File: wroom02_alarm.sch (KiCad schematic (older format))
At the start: 29 parts, among them J1 Serial, J10 pin, J11 pin, J2 BARREL_JACK, J3 microUSB, J4 pin, J5 pin, J6 pin, J7 pin, J8 pin, J9 pin, Q1 Q_NMOS_GDS, SW1 Write, SW2 RESET, U1 wroom02, U3 7803

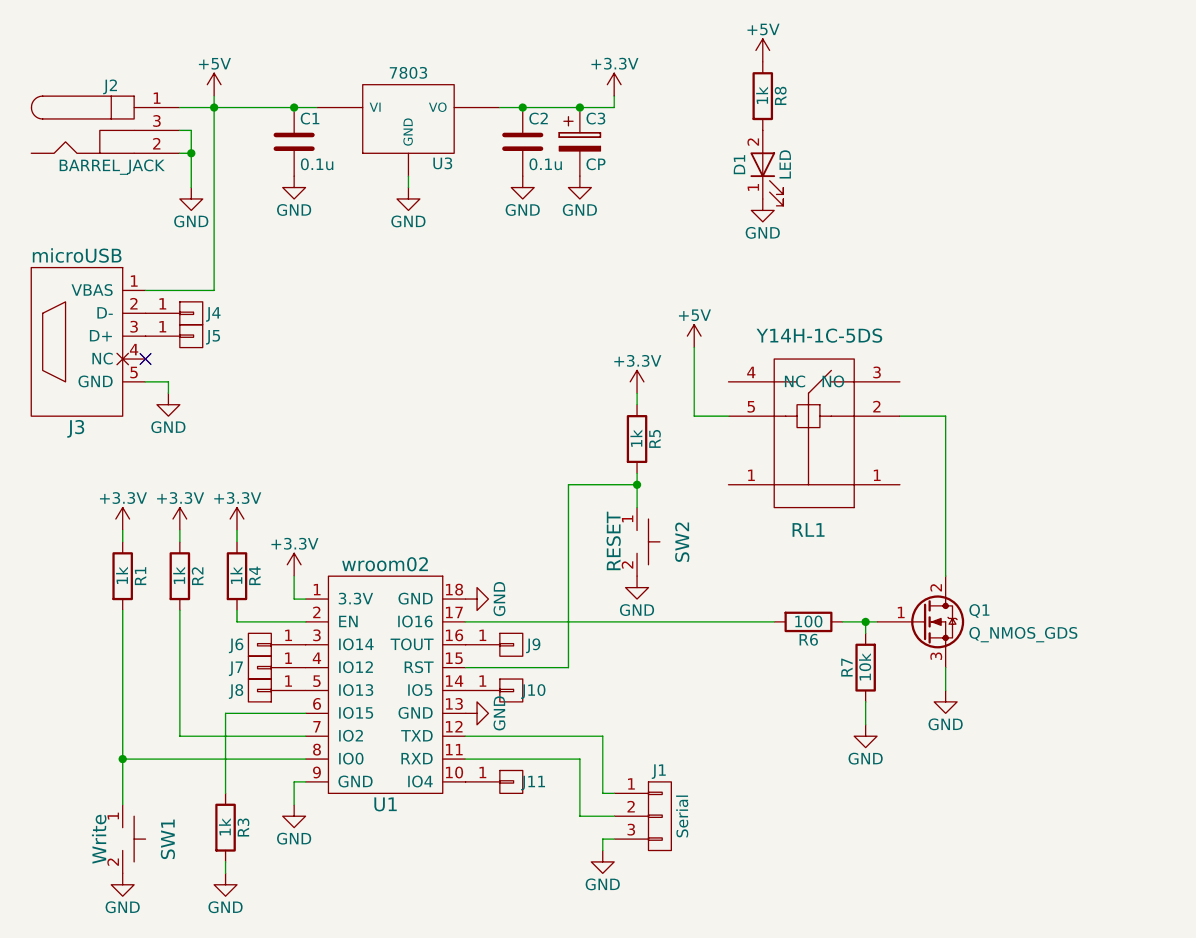
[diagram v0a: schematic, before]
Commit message: 基板も完成
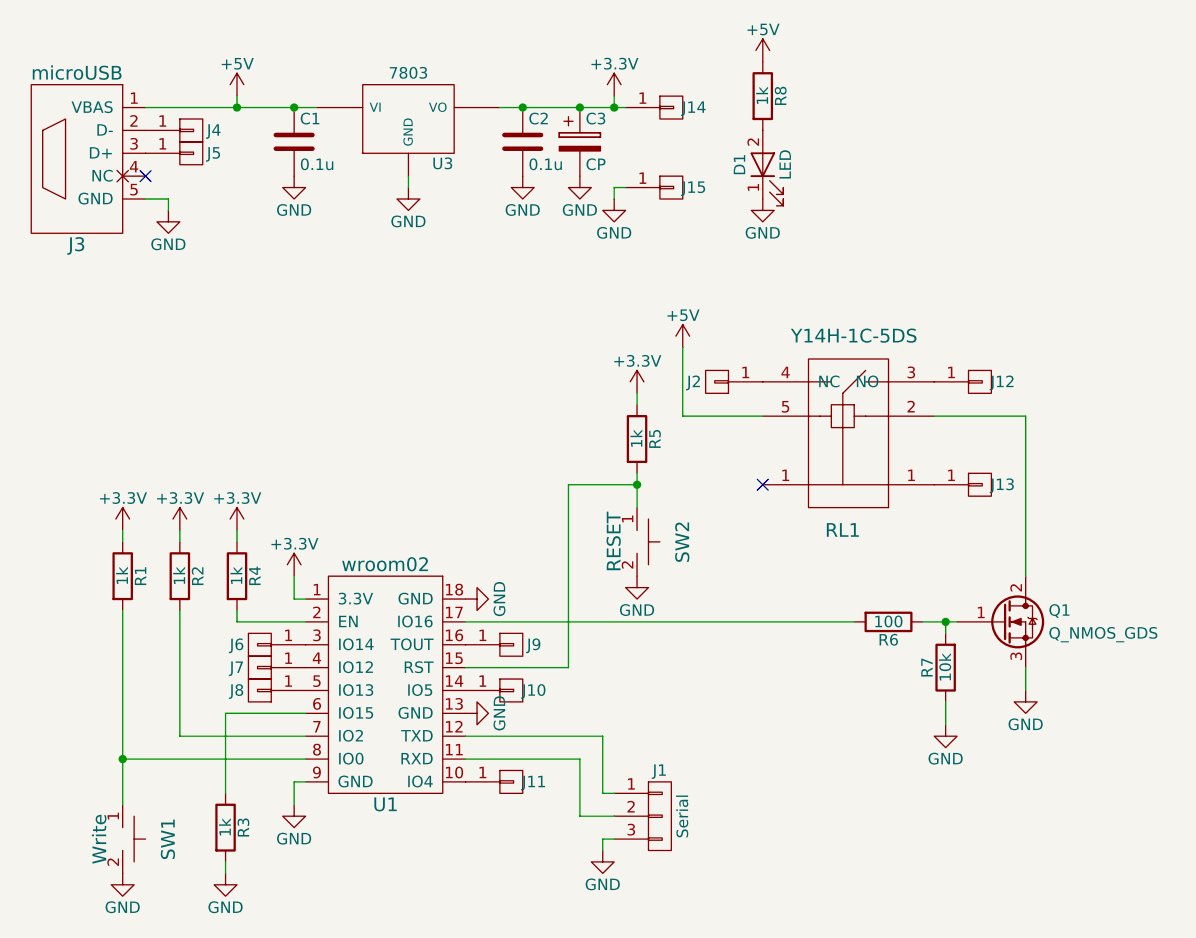
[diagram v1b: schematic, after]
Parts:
- removed J2: BARREL_JACK, symbol BARREL_JACK
- added J12, J13, J14, J15, J2: pin, pad:universal, symbol CONN_01X01
- C1, C2: footprint (none) -> Capacitors_SMD:C_0603_HandSoldering
- C3: footprint (none) -> Capacitors_THT:CP_Radial_D8.0mm_P2.50mm
- D1: footprint (none) -> LEDs:LED_0603_HandSoldering
- J1: footprint (none) -> Pin_Headers:Pin_Header_Straight_1x03_Pitch2.54mm
- J10, J11, J4, J5, J6, J7, J8, J9: footprint (none) -> pad:universal
- J3: footprint (none) -> lib:microUSB
- Q1: footprint (none) -> TO_SOT_Packages_THT:TO-220_Vertical
- R1, R2, R3, R4, R5, R6, R7, R8: footprint (none) -> Resistors_SMD:R_0603_HandSoldering
- RL1: footprint (none) -> lib:Y14H-1C-5DS
- SW1, SW2: footprint (none) -> lib:switch
- U1: footprint (none) -> lib:WROOM02
- U3: footprint (none) -> TO_SOT_Packages_SMD:TO-252-3_TabPin2
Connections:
- net +3V3: now also J14.1 (P1)
- net GND: now also J15.1 (P1)
- net at RL1.1: now also J13.1 (P1)
- net at RL1.3 (NO): now also J12.1 (P1)
- net at RL1.4 (NC): now also J2.1 (P1)
- no-connect marks 1 -> 2
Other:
- moved on the sheet: J3, J4, J5, Q1, R6, R7, RL1
